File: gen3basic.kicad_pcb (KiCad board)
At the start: 2 copper layers, 35 parts, among them J1 AVR-ISP-6, J2 Screw_Terminal_01x02, J3 Conn_01x08, J4 Conn_01x08, J5 Conn_01x08, J6 Screw_Terminal_01x04, U1 ATMEGA328-PU, Y1 Resonator

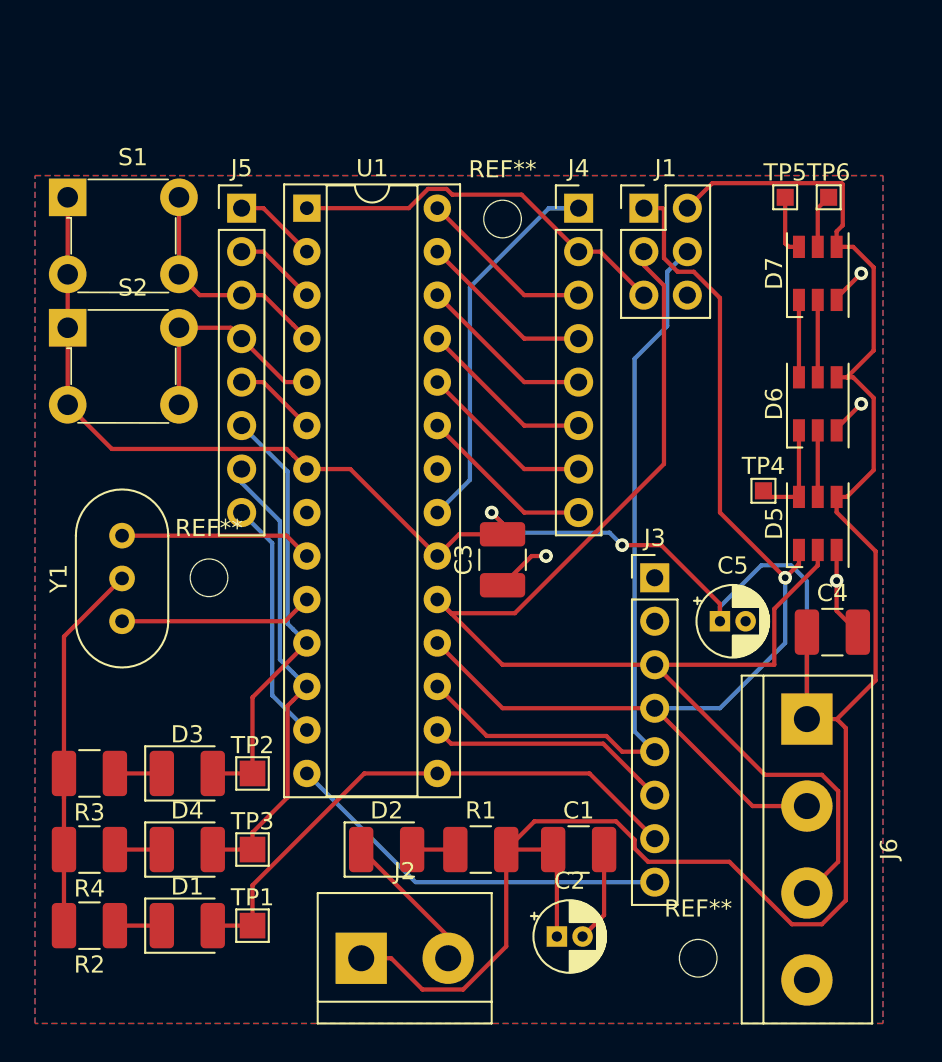
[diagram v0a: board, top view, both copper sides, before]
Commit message: moved a bunch of stuff around.
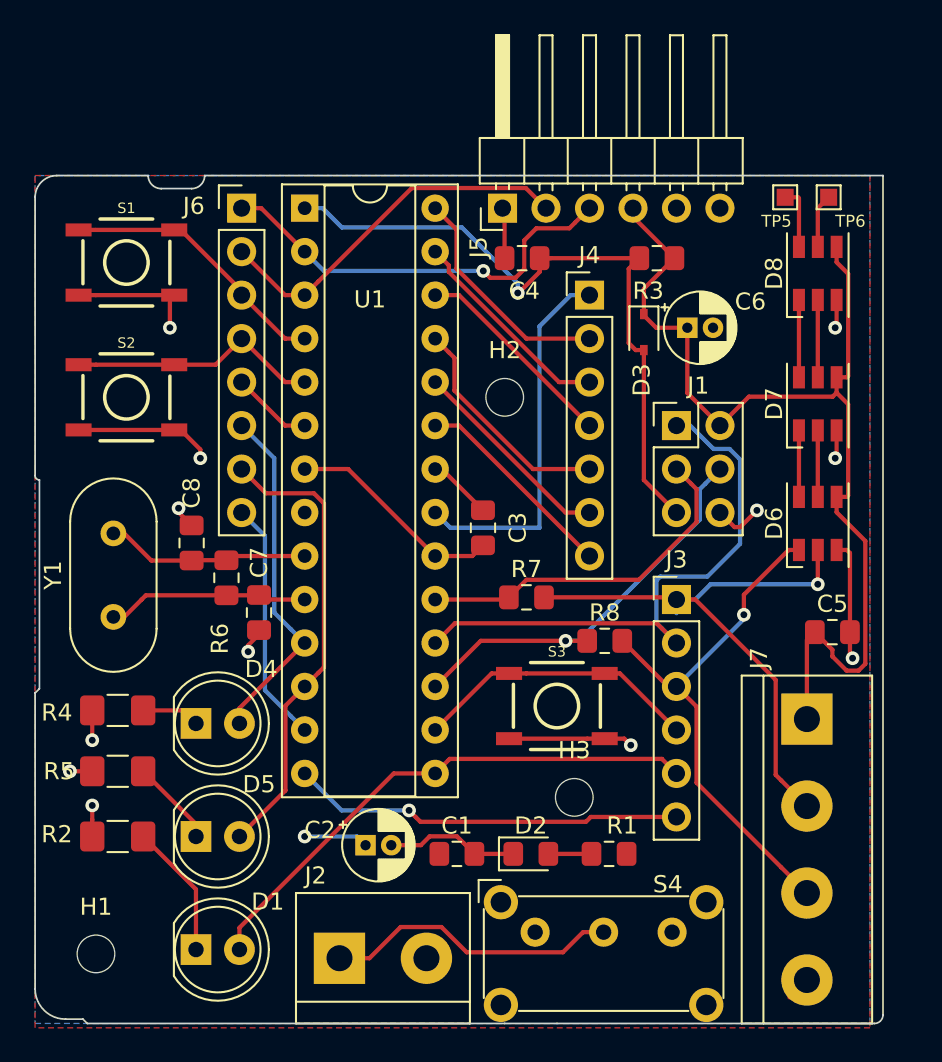
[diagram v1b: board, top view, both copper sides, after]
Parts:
- removed REF** (x3): MountingHole_2.2mm_M2_DIN965, MountingHole:MountingHole_2.2mm_M2_DIN965
- removed TP1, TP2, TP3: TestPoint, TestPoint:TestPoint_Pad_1.5x1.5mm
- removed TP4: TestPoint, TestPoint:TestPoint_Pad_1.0x1.0mm
- added C4: 100 nF, Capacitor_SMD:C_0805_2012Metric_Pad1.15x1.40mm_HandSolder, F.Cu at (79.2, 49.3)
- added C7: 22pF, Capacitor_SMD:C_0805_2012Metric_Pad1.15x1.40mm_HandSolder, F.Cu at (63.9, 70.0)
- added C8: 22pF, Capacitor_SMD:C_0805_2012Metric_Pad1.15x1.40mm_HandSolder, F.Cu at (59.9, 65.9)
- added D3: 1N4148WS, Diode_SMD:D_SOD-323, F.Cu at (86.4, 53.6)
- added H1: MountingHole, MountingHole:MountingHole_2.2mm_M2_ISO7380, F.Cu at (54.4, 89.9)
- added H2: MountingHole, MountingHole:MountingHole_2.2mm_M2_ISO7380, F.Cu at (78.2, 57.4)
- added H3: MountingHole, MountingHole:MountingHole_2.2mm_M2_ISO7380, F.Cu at (82.3, 80.8)
- added J5: Conn_01x06, Connector_PinHeader_2.54mm:PinHeader_1x06_P2.54mm_Horizontal, F.Cu at (78.1, 46.4)
- added R3: 10k, Resistor_SMD:R_0805_2012Metric_Pad1.15x1.40mm_HandSolder, F.Cu at (87.1, 49.3)
- added R6: 1M, Resistor_SMD:R_0805_2012Metric_Pad1.15x1.40mm_HandSolder, F.Cu at (62.0, 67.9)
- added R7: 330k, Resistor_SMD:R_0805_2012Metric_Pad1.15x1.40mm_HandSolder, F.Cu at (79.5, 69.1)
- added R8: 330k, Resistor_SMD:R_0805_2012Metric_Pad1.15x1.40mm_HandSolder, F.Cu at (84.1, 71.6)
- added S3: MOMENTARY-SWITCH-SPST-SMD-5.2-REDUNDANT, SparkFun-Switches:TACTILE_SWITCH_SMD_5.2MM, F.Cu at (81.3, 75.4)
- added S4: EG1224, Button_Switch_THT:SW_E-Switch_EG1224_SPDT_Angled, F.Cu at (80.0, 88.6)
- C1: footprint Capacitor_SMD:C_1210_3225Metric_Pad1.42x2.65mm_HandSolder -> Capacitor_SMD:C_0805_2012Metric_Pad1.15x1.40mm_HandSolder
- C3: value C -> 100 nF; footprint Capacitor_SMD:C_1210_3225Metric_Pad1.42x2.65mm_HandSolder -> Capacitor_SMD:C_0805_2012Metric_Pad1.15x1.40mm_HandSolder
- C5: renamed from C4; value C -> 100 nF; footprint Capacitor_SMD:C_1210_3225Metric_Pad1.42x2.65mm_HandSolder -> Capacitor_SMD:C_0805_2012Metric_Pad1.15x1.40mm_HandSolder
- D1: footprint LED_SMD:LED_1210_3225Metric_Pad1.42x2.65mm_HandSolder -> LED_THT:LED_D5.0mm_Clear
- D2: footprint LED_SMD:LED_1210_3225Metric_Pad1.42x2.65mm_HandSolder -> LED_SMD:LED_0805_2012Metric_Pad1.15x1.40mm_HandSolder
- D4: renamed from D3; footprint LED_SMD:LED_1210_3225Metric_Pad1.42x2.65mm_HandSolder -> LED_THT:LED_D5.0mm_Clear
- D5: renamed from D4; footprint LED_SMD:LED_1210_3225Metric_Pad1.42x2.65mm_HandSolder -> LED_THT:LED_D5.0mm_Clear
- J3: value Conn_01x08 -> Conn_01x06; footprint Connector_PinHeader_2.54mm:PinHeader_1x08_P2.54mm_Vertical -> Connector_PinHeader_2.54mm:PinHeader_1x06_P2.54mm_Vertical
- J4: value Conn_01x08 -> Conn_01x07; footprint Connector_PinHeader_2.54mm:PinHeader_1x08_P2.54mm_Vertical -> Connector_PinHeader_2.54mm:PinHeader_1x07_P2.54mm_Vertical
- R1: footprint Resistor_SMD:R_1210_3225Metric_Pad1.42x2.65mm_HandSolder -> Resistor_SMD:R_0805_2012Metric_Pad1.15x1.40mm_HandSolder
- R2: footprint Resistor_SMD:R_1210_3225Metric_Pad1.42x2.65mm_HandSolder -> Resistor_SMD:R_1206_3216Metric_Pad1.42x1.75mm_HandSolder
- R4: renamed from R3; footprint Resistor_SMD:R_1210_3225Metric_Pad1.42x2.65mm_HandSolder -> Resistor_SMD:R_1206_3216Metric_Pad1.42x1.75mm_HandSolder
- R5: renamed from R4; footprint Resistor_SMD:R_1210_3225Metric_Pad1.42x2.65mm_HandSolder -> Resistor_SMD:R_1206_3216Metric_Pad1.42x1.75mm_HandSolder
- S1, S2: value 1825910-6 -> MOMENTARY-SWITCH-SPST-SMD-5.2-REDUNDANT; footprint digikey-footprints:Switch_Tactile_THT_6x6mm -> SparkFun-Switches:TACTILE_SWITCH_SMD_5.2MM
- Y1: value Resonator -> 16.0000MHZ 20PF; footprint Crystal:Resonator-3Pin_W10.0mm_H5.0mm -> Crystal:Crystal_HC49-U_Vertical
- moved C6 17.3 mm to (88.9, 53.3)
- moved J1 12.8 mm to (88.3, 59.1)
- moved C2 12.4 mm to (70.1, 83.6)
- moved D2 8.42 mm to (79.8, 84.1)
- moved R1 7.50 mm to (84.3, 84.1)
- moved C1 7.12 mm to (75.4, 84.1)
- moved R2 5.46 mm to (55.6, 83.1)
- moved S2 5.32 mm to (56.1, 57.4)
- moved S1 5.13 mm to (56.1, 49.5)
- moved J4 5.12 mm to (83.2, 51.4)
- moved R5 4.86 mm to (55.6, 79.2)
- moved R4 4.04 mm to (55.6, 75.7)
- moved D4 2.96 mm to (60.2, 76.5)
- moved C3 2.19 mm to (77.0, 65.0)
- moved J3 1.80 mm to (88.3, 69.2)
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- renumbered C5 to C6, D5 to D6, D6 to D7, D7 to D8, J5 to J6, J6 to J7
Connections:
- net /PD0 renamed /PD0-RXD
- net /PD1 renamed /PD1-TXD
- C3 pad 1: GND -> VCC
- C3 pad 2: VCC -> GND
- D6 pad 1: /MISO -> /APA-DI
- D6 pad 2: /PB5 -> /APA-CI
- J1 pad 5: /PC6 -> /RESET#
- J2 pad 1: VCC -> /IN+
- J3 pad 1: GND -> /APA-CI
- J3 pad 2: GND -> /MISO
- J3 pad 3: /PB5 -> /APA-DI
- J3 pad 4: /MISO -> /PB2
- J3 pad 5: /MOSI -> /LED1
- J3 pad 6: /PB2 -> /PB0
- J4 pad 2: /PC6 -> /PC5
- J4 pad 3: /PC5 -> /PC4
- J4 pad 4: /PC4 -> /PC3
- J4 pad 5: /PC3 -> /PC2
- J4 pad 6: /PC2 -> /PC1
- J4 pad 7: /PC1 -> /PC0
- J7 pad 2: /MISO -> /APA-CI
- J7 pad 3: /PB5 -> /APA-DI
- S1 pad 1: VCC -> /PD2
- S1 pad 3: VCC -> GND
- S1 pad 4: /PD2 -> GND
- S2 pad 1: VCC -> /PD3
- S2 pad 3: VCC -> GND
- S2 pad 4: /PD3 -> GND
- U1 pad 1: /PC6 -> /RESET#
- Y1 pad 2: GND -> OSC2
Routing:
- net VCC: track 188.3 -> 78.1 mm, vias 2 -> 1
- net /PB5: track 79.6 -> 20.7 mm
- net /RESET#: track 0.00 -> 41.4 mm, vias 0 -> 1
- net /APA-CI: track 0.00 -> 35.8 mm, vias 0 -> 1
- net /MISO: track 66.8 -> 35.1 mm, vias 1 -> 0
- net /APA-DI: track 0.00 -> 31.2 mm, vias 0 -> 1
- net /PC6: track 22.7 -> 0.00 mm
- net /MOSI: track 45.3 -> 24.2 mm, vias 0 -> 1
- net /PD0-RXD: track 4.86 -> 24.7 mm, vias 0 -> 1
- net /IN+: track 0.00 -> 17.3 mm
- net /PD1-TXD: track 4.86 -> 21.9 mm
- net GND: track 50.7 -> 56.5 mm, vias 4 -> 12
- net Net-(D1-Pad1): track 2.96 -> 8.38 mm
- net /LED2: track 25.5 -> 20.5 mm
- net /PC5: track 9.72 -> 13.5 mm
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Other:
- board outline added: 49.5 x 49.5 mm
